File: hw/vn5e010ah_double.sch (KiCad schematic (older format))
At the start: 6 parts, among them U701 VN5E010AH, U702 VN5E010AH

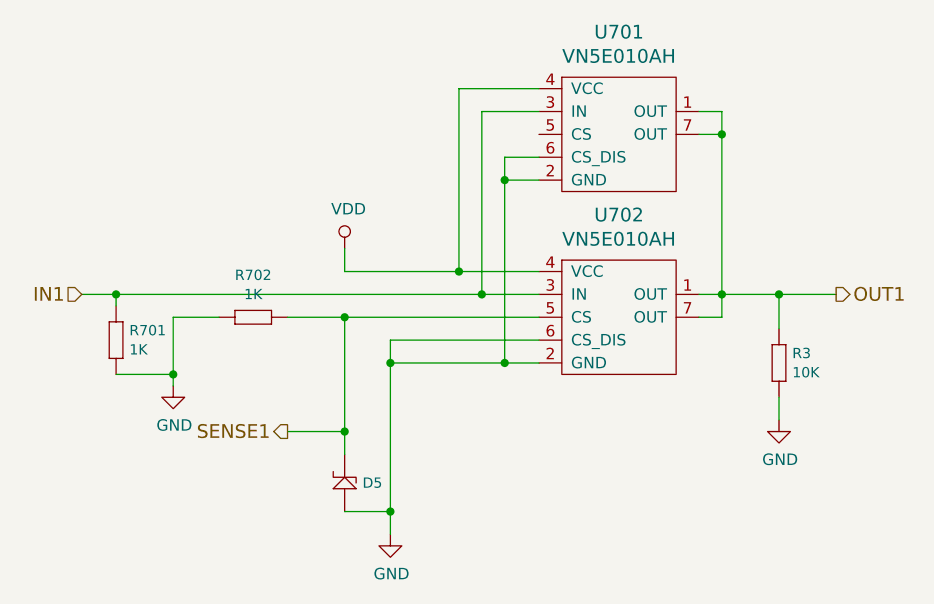
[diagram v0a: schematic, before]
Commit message: pcb 3.6.0 created, with double fets in work & drive lights
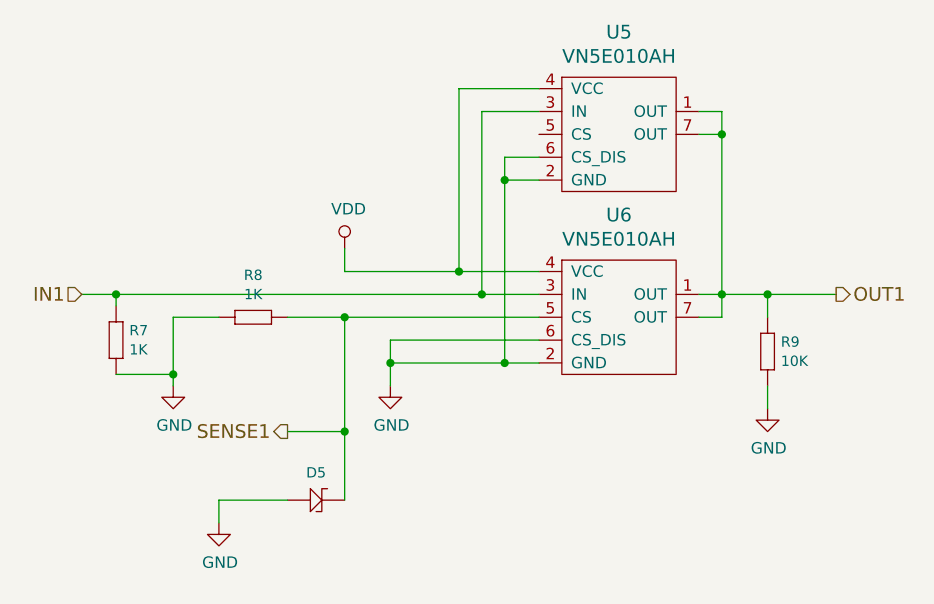
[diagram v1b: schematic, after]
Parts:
- removed D5: ZENER_MM3Z3V6T1G, usevolt:SOD-323, symbol usevolt:ZENER_MM3Z3V6T1G
- removed R3: 10K, yageo:0603, symbol yageo:10K
- removed R702: 1K, yageo:0603, symbol yageo:1K
- added D8: ZENER_MM3Z3V6T1G, usevolt:SOD-323, symbol usevolt:ZENER_MM3Z3V6T1G
- added R1203: 1K, yageo:0603, symbol yageo:1K
- added R6: 10K, yageo:0603, symbol yageo:10K
- renumbered R701 to R1, U701 to U1201, U702 to U1202
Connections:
- net GND: now also D8.2, R1203.2 (R2), R6.1 (R1)
- net OUT1: now also R6.2 (R2)
- net SENSE1: now also D8.1, R1203.1 (R1)
